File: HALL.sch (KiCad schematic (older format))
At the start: 1 part, among them P6 CON_HALL

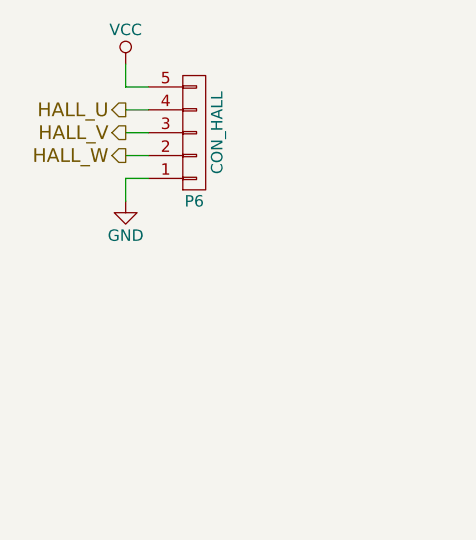
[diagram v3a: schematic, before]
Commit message: i think im good with the schematics
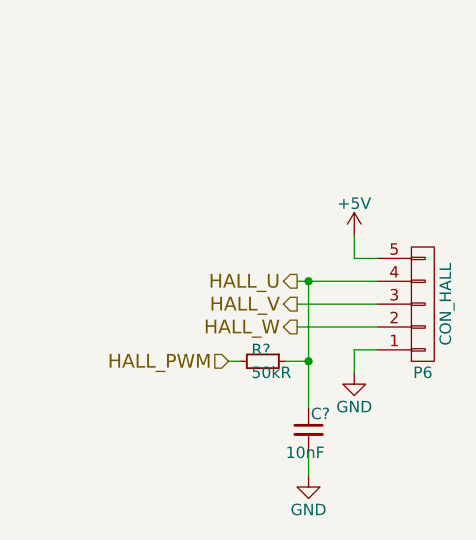
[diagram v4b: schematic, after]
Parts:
- added C?: 10nF, symbol C_Small
- added R?: 50kR, symbol R_Small
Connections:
- net GND: now also C?.2
- net HALL_U: now also C?.1, R?.1
- net VCC renamed +5V
- new net HALL_PWM: R?.2
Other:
- moved on the sheet: P6
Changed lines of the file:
@@
 $Descr A4 11693 8268
 encoding utf-8
-Sheet 12 12
+Sheet 9 12
 Title ""
 Date ""
@@
 L CONN_01X05 P6
 U 1 1 57ADAAC3
-P 1300 950
-F 0 "P6" H 1300 1250 50  0000 C CNN
-F 1 "CON_HALL" V 1400 950 50  0000 C CNN
-F 2 "Terminal_Blocks:TerminalBlock_Pheonix_MPT-2.54mm_5pol" H 1300 950 50  0001 C CNN
-F 3 "" H 1300 950 50  0000 C CNN
-	1    1300 950
+P 2300 1700
+F 0 "P6" H 2300 2000 50  0000 C CNN
+F 1 "CON_HALL" V 2400 1700 50  0000 C CNN
+F 2 "Terminal_Blocks:TerminalBlock_Pheonix_MPT-2.54mm_5pol" H 2300 1700 50  0001 C CNN
+F 3 "" H 2300 1700 50  0000 C CNN
+	1    2300 1700
 	1    0    0    1
 $EndComp
 Wire Wire Line
-	1000 650  1000 750
+	2000 1400 2000 1500
 Wire Wire Line
-	1000 750  1100 750
+	2000 1500 2100 1500
 $Comp
 L GND #PWR049
 U 1 1 57ADAB3C
-P 1000 1250
-F 0 "#PWR049" H 1000 1000 50  0001 C CNN
-F 1 "GND" H 1000 1100 50  0000 C CNN
-F 2 "" H 1000 1250 50  0000 C CNN
-F 3 "" H 1000 1250 50  0000 C CNN
-	1    1000 1250
+P 2000 2000
+F 0 "#PWR049" H 2000 1750 50  0001 C CNN
+F 1 "GND" H 2000 1850 50  0000 C CNN
+F 2 "" H 2000 2000 50  0000 C CNN
+F 3 "" H 2000 2000 50  0000 C CNN
+	1    2000 2000
 	1    0    0    -1
 $EndComp
 Wire Wire Line
-	1000 1250 1000 1150
+	2000 2000 2000 1900
 Wire Wire Line
-	1000 1150 1100 1150
-Text HLabel 1000 850  0    60   Output ~ 0
+	2000 1900 2100 1900
+Text HLabel 1750 1600 0    60   Output ~ 0
 HALL_U
-Text HLabel 1000 950  0    60   Output ~ 0
+Text HLabel 1750 1700 0    60   Output ~ 0
 HALL_V
-Text HLabel 1000 1050 0    60   Output ~ 0
+Text HLabel 1750 1800 0    60   Output ~ 0
 HALL_W
-Wire Wire Line
-	1000 1050 1100 1050
-Wire Wire Line
-	1100 950  1000 950
-Wire Wire Line
-	1000 850  1100 850
 $Comp
-L VCC #PWR050
-U 1 1 57B357EE
-P 1000 650
-F 0 "#PWR050" H 1000 500 50  0001 C CNN
-F 1 "VCC" H 1000 800 50  0000 C CNN
-F 2 "" H 1000 650 50  0000 C CNN
-F 3 "" H 1000 650 50  0000 C CNN
-	1    1000 650
+L +5V #PWR?
+U 1 1 580F5FAC
+P 2000 1400
+F 0 "#PWR?" H 2000 1250 50  0001 C CNN
+F 1 "+5V" H 2000 1540 50  0000 C CNN
+F 2 "" H 2000 1400 50  0000 C CNN
+F 3 "" H 2000 1400 50  0000 C CNN
+	1    2000 1400
 	1    0    0    -1
 $EndComp
+$Comp
+L C_Small C?
+U 1 1 580F6E53
+P 1800 2250
+F 0 "C?" H 1810 2320 50  0000 L CNN
+F 1 "10nF" H 1700 2150 50  0000 L CNN
+F 2 "" H 1800 2250 50  0000 C CNN
+F 3 "" H 1800 2250 50  0000 C CNN
+	1    1800 2250
+	1    0    0    -1
+$EndComp
+$Comp
+L GND #PWR?
+U 1 1 580F6E9B
+P 1800 2450
+F 0 "#PWR?" H 1800 2200 50  0001 C CNN
+F 1 "GND" H 1800 2300 50  0000 C CNN
+F 2 "" H 1800 2450 50  0000 C CNN
+F 3 "" H 1800 2450 50  0000 C CNN
+	1    1800 2450
+	1    0    0    -1
+$EndComp
+$Comp
+L R_Small R?
+U 1 1 580F71C7
+P 1600 1950
+F 0 "R?" V 1550 1900 50  0000 L CNN
+F 1 "50kR" V 1650 1900 50  0000 L CNN
+F 2 "" H 1600 1950 50  0000 C CNN
+F 3 "" H 1600 1950 50  0000 C CNN
+	1    1600 1950
+	0    1    1    0
+$EndComp
+Wire Wire Line
+	1750 1600 2100 1600
+Wire Wire Line
+	1750 1700 2100 1700
+Wire Wire Line
+	1750 1800 2100 1800
+Wire Wire Line
+	1800 2350 1800 2450
+Text HLabel 1450 1950 0    60   Input ~ 0
+HALL_PWM
+Wire Wire Line
+	1450 1950 1500 1950
+Wire Wire Line
+	1700 1950 1800 1950
+Wire Wire Line
+	1800 1600 1800 2150
+Connection ~ 1800 1600
+Connection ~ 1800 1950
 $EndSCHEMATC
